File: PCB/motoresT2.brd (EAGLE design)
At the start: 102.5 x 91.4 mm, 11 parts

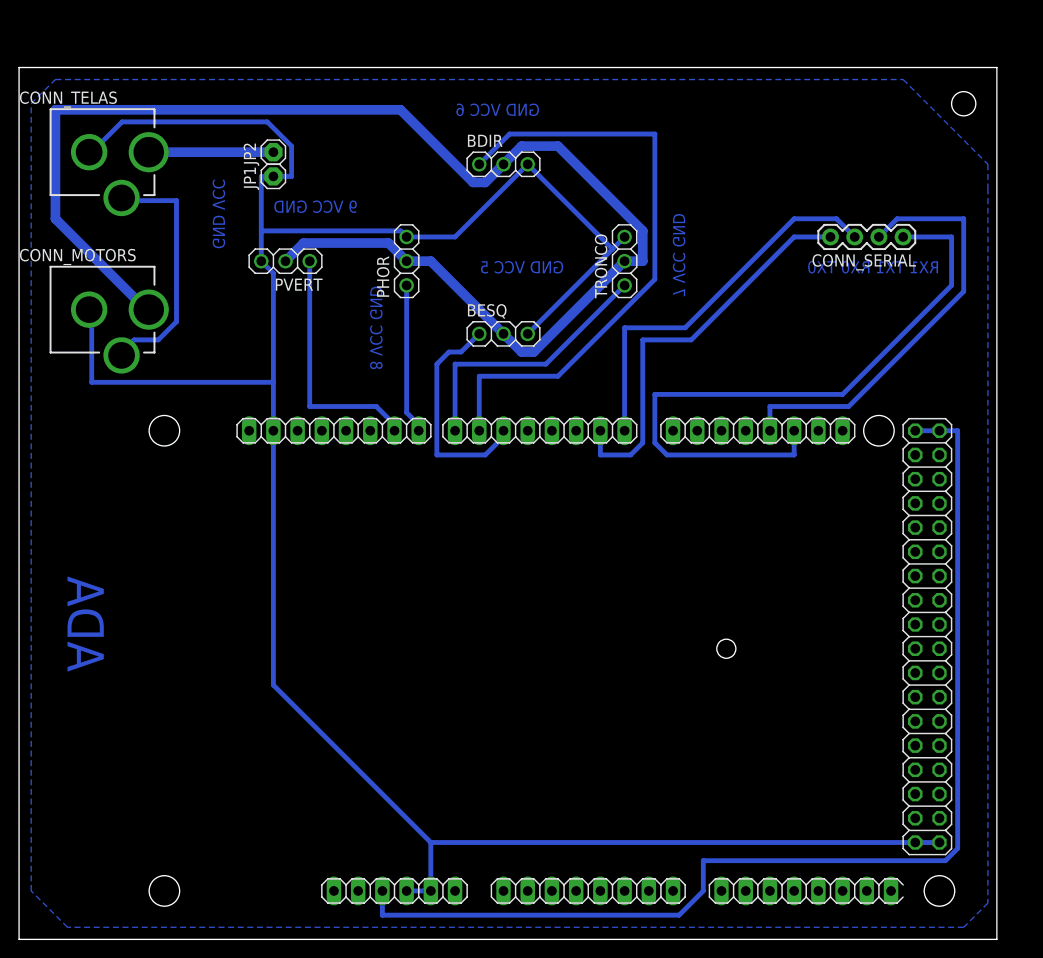
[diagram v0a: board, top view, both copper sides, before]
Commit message: PCD motores arrumada
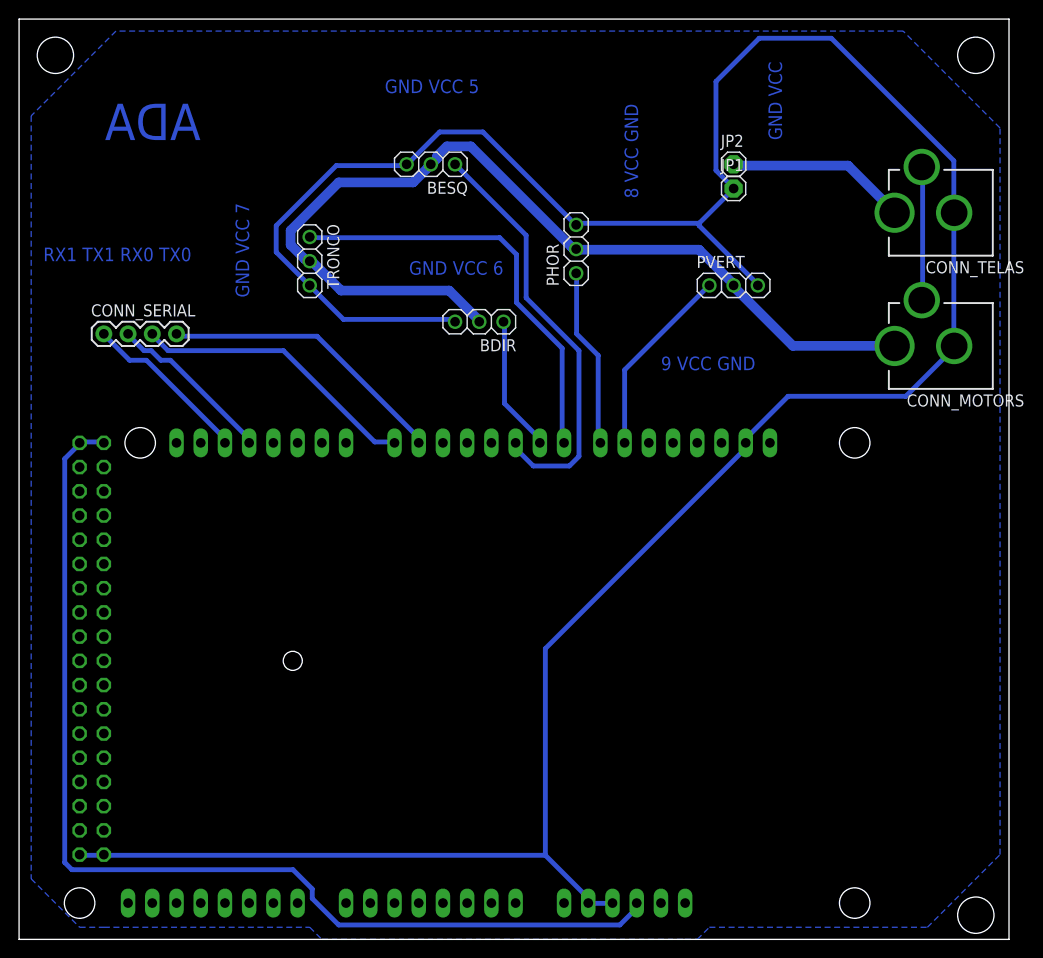
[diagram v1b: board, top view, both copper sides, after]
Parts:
- moved CONN_TELAS 105.6 mm to (105.4, 76.2), turned to 90 degrees
- moved CONN_MOTORS 105.5 mm to (105.4, 62.2), turned to 90 degrees
- moved MEGA 102.9 mm to (102.9, 1.27), flipped to the bottom
- moved CONN_SERIAL 84.4 mm to (8.89, 63.5), turned to 0 degrees
- moved JP1 48.3 mm to (74.9, 78.7), turned to 0 degrees
- moved JP2 48.3 mm to (74.9, 81.3), turned to 0 degrees
- moved PVERT 47.1 mm to (74.9, 68.6), turned to 0 degrees
- moved TRONCO 33.0 mm to (30.5, 71.1), turned to 270 degrees
- moved BESQ 19.3 mm to (43.2, 81.3), turned to 180 degrees
- moved PHOR 17.8 mm to (58.4, 72.4)
- moved BDIR 16.7 mm to (48.3, 64.8), turned to 180 degrees
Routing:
- net RX1: track 68.8 -> 17.7 mm
- net N$1: track 63.3 -> 14.4 mm
- net VCC1: track 145.3 -> 100.8 mm
- net GND: track 253.4 -> 291.7 mm
- net TX1: track 45.2 -> 17.7 mm
- net N$6: track 23.7 -> 44.4 mm
- net N$2: track 28.2 -> 44.3 mm
- net GNDBREAK: track 26.1 -> 14.1 mm
- net TX0: track 42.5 -> 30.5 mm
- net RX0: track 40.4 -> 30.2 mm
- net VCC2: track 13.1 -> 19.0 mm
- net N$5: track 25.6 -> 20.2 mm
- net +5V: track 115.9 -> 111.8 mm
- net N$4: track 15.8 -> 18.9 mm
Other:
- board size 102.5 x 91.4 mm -> 103.8 x 96.5 mm
- board text added: "GND VCC 7"
- board text removed: "7 VCC GND"
